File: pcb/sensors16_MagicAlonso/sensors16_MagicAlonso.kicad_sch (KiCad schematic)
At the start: 64 parts, among them J1 Sensors, U1 QRE1113GR, U10 QRE1113GR, U11 QRE1113GR, U12 QRE1113GR, U13 QRE1113GR, U14 QRE1113GR, U15 QRE1113GR, U16 QRE1113GR, U2 QRE1113GR, U20 CD74HC4067, U3 QRE1113GR, U30 CD74HC4067M, U4 QRE1113GR, U5 QRE1113GR, U6 QRE1113GR, U7 QRE1113GR, U8 QRE1113GR, U9 QRE1113GR

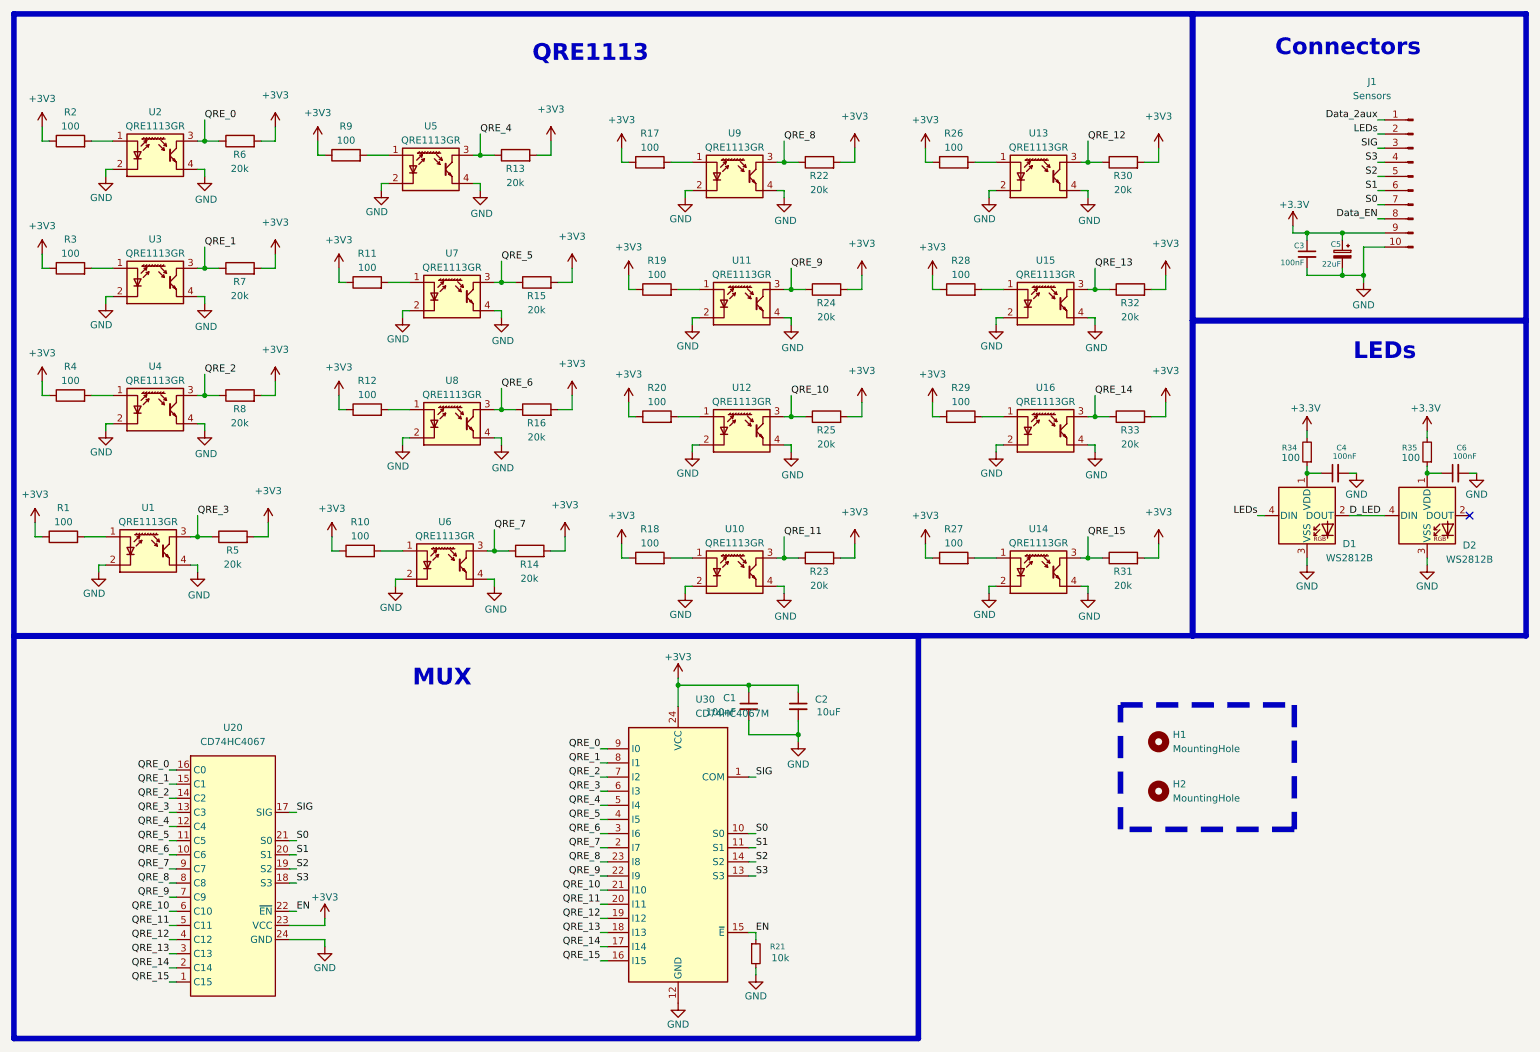
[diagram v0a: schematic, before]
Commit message: sensors16 pcb update
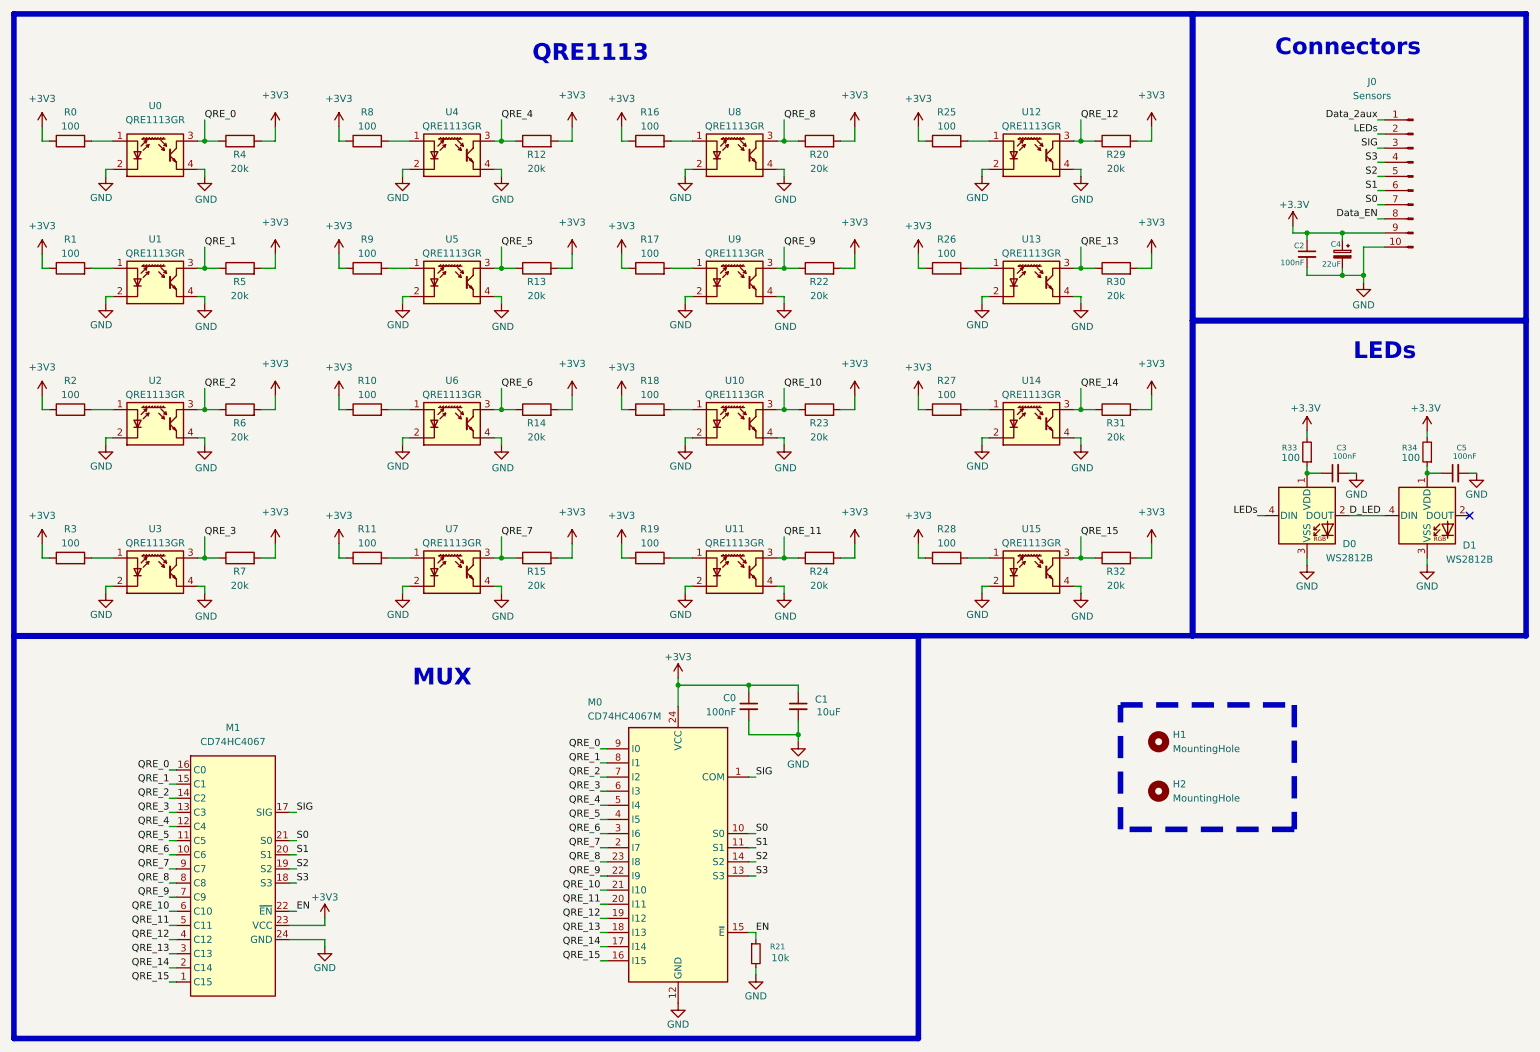
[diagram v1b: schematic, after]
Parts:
- renumbered C1 to C0, C2 to C1, C3 to C2, C4 to C3, C5 to C4, C6 to C5, D1 to D0, D2 to D1, J1 to J0, U30 to M0, U20 to M1, R2 to R0, R3 to R1, R12 to R10, R10 to R11, R13 to R12, R15 to R13, R16 to R14, R14 to R15, R17 to R16, R19 to R17, R20 to R18, R18 to R19, R4 to R2, R22 to R20, R24 to R22, R25 to R23, R23 to R24, R26 to R25, R28 to R26, R29 to R27, R27 to R28, R30 to R29, R1 to R3, R32 to R30, R33 to R31, R31 to R32, R34 to R33, R35 to R34, R6 to R4, R7 to R5, R8 to R6, R5 to R7, R9 to R8, R11 to R9, U2 to U0, U3 to U1, U12 to U10, U10 to U11, U13 to U12, U15 to U13, U16 to U14, U14 to U15, U4 to U2, U1 to U3, U5 to U4, U7 to U5, U8 to U6, U6 to U7, U9 to U8, U11 to U9
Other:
- moved on the sheet: R11, R12, R13, R15, R16, R17, R18, R2, R20, R22, R23, R25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
